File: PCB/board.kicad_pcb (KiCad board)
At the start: 2 copper layers, 161 parts, among them J1 Micro_SD_Card, J10 Conn_01x10, J11 Conn_01x02, J12 Conn_02x04_Odd_Even, J13 Conn_01x02, J14 Conn_01x02, J15 Conn_01x03, J16 Conn_01x02, J17 Conn_01x05, J18 Conn_01x04, J19 Conn_01x04, J2 Conn_ARM_JTAG_SWD_10, J20 Conn_01x02, J21 Conn_01x03, J22 Conn_02x04_Odd_Even, J23 Conn_01x04, J24 Conn_01x04, J25 Conn_01x02, J26 Conn_01x03, J27 Conn_02x04_Odd_Even, J28 Conn_01x04, J29 Conn_01x04, J3 USB_C_Receptacle_USB2.0_14P, J30 Conn_01x02, J31 Conn_01x03, J32 Conn_01x02, J33 Conn_01x02, J34 Conn_01x02, J35 Conn_01x02, J36 Conn_01x02, J37 Conn_01x02, J4 Conn_01x04, J5 Conn_01x04, J6 Conn_01x02, J7 Conn_01x03, J8 Conn_02x04_Odd_Even, J9 Conn_01x10, Q1 IRLML6402, Q2 NMOS, Q3 NMOS, Q4 NMOS, Q5 NMOS, Q6 NMOS, SW1 SW_Push, SW2 SW_Push, U1 STM32H743VITx, U2 AP7361C, U4 TMC Stepstick, U5 TMC Stepstick, U6 TMC Stepstick, U7 TMC Stepstick, U8 AP63203WU, Y2 25 MHz

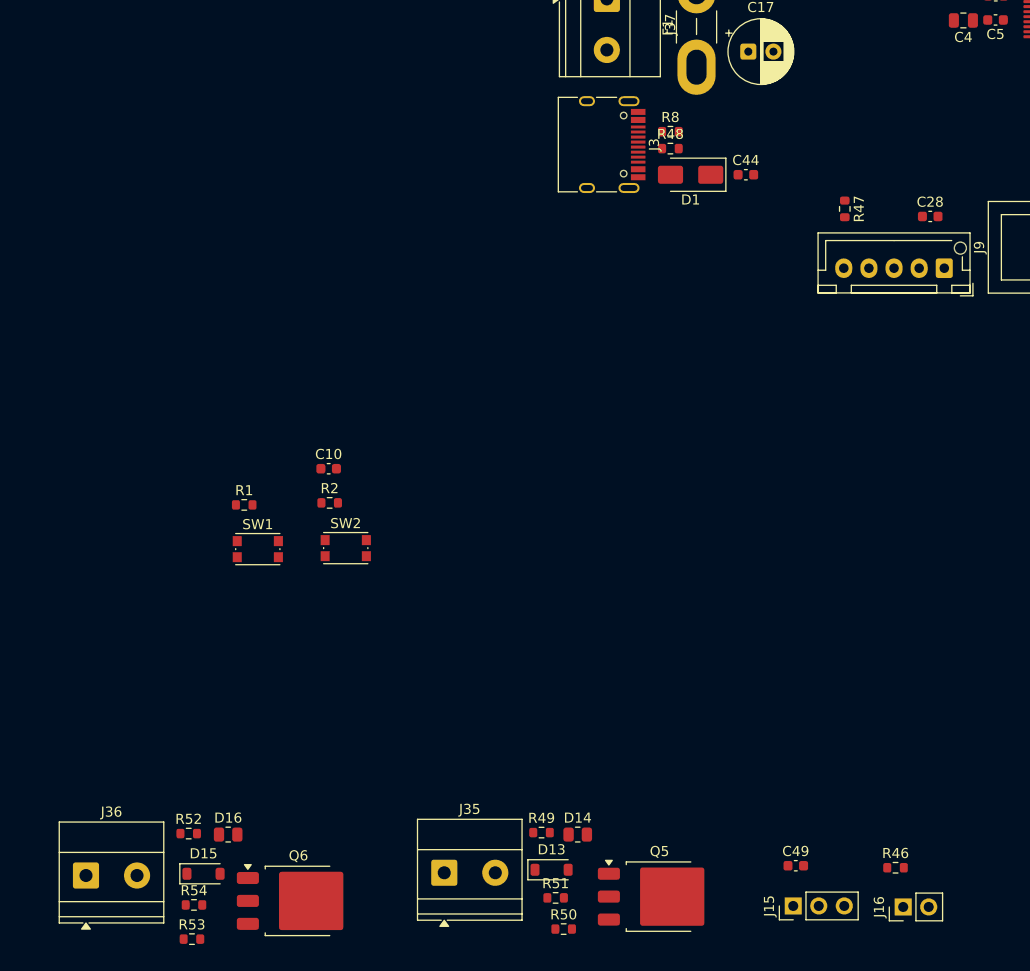
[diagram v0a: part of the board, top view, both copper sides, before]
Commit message: heaters
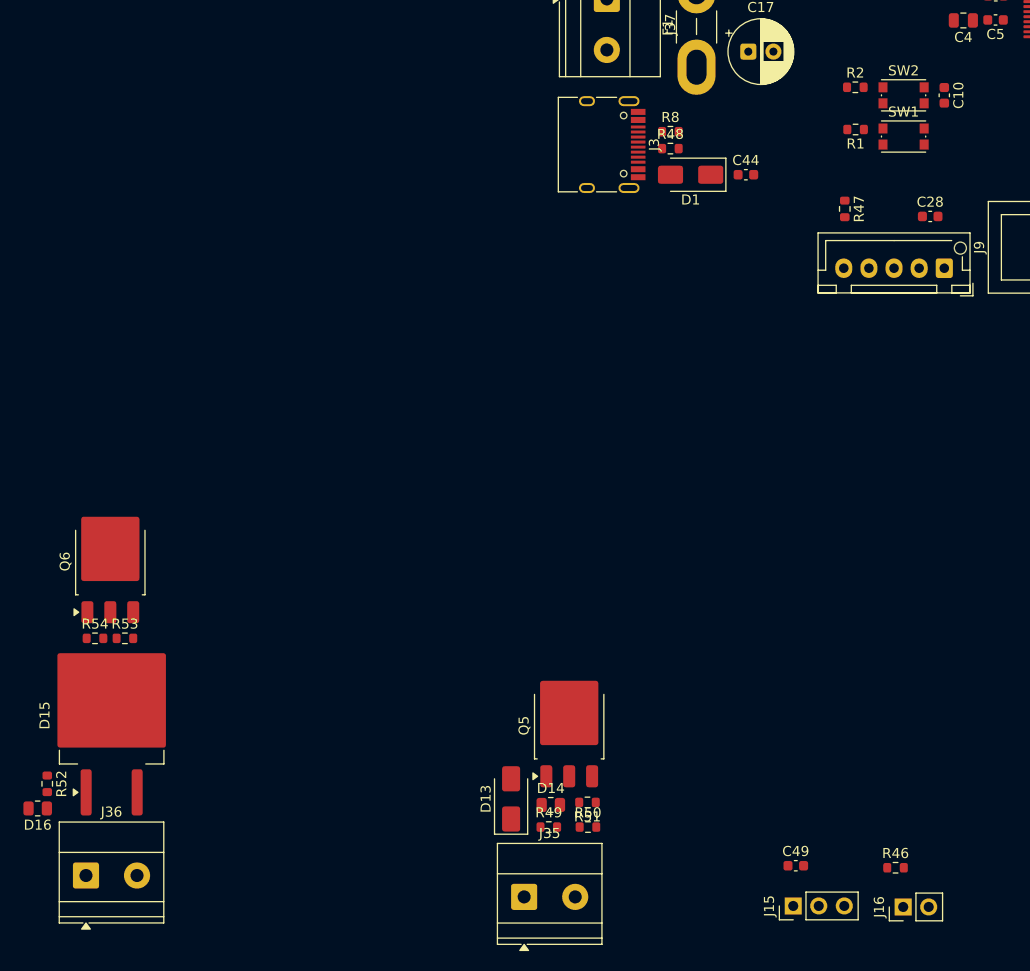
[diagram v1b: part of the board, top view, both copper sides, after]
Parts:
- D13: footprint Diode_SMD:D_SOD-123 -> Diode_SMD:D_SMA
- D15: footprint Diode_SMD:D_SOD-123 -> Package_TO_SOT_SMD:TO-263-2
- moved SW1 76.2 mm to (170.7, 107.8)
- moved C10 71.6 mm to (174.8, 103.8), turned to -90 degrees
- moved SW2 71.5 mm to (170.7, 103.8)
- moved R1 71.4 mm to (165.9, 107.2), turned to 180 degrees
- moved R2 66.7 mm to (165.9, 103.0)
- moved Q6 38.6 mm to (91.8, 150.1), turned to 90 degrees
- moved R53 30.7 mm to (93.2, 157.8)
- moved R54 28.3 mm to (90.3, 157.8)
- moved Q5 19.2 mm to (137.4, 166.5), turned to 90 degrees
- moved D16 19.1 mm to (84.5, 174.7), turned to 180 degrees
- moved D15 18.2 mm to (91.9, 165.4), turned to 90 degrees
- moved R52 14.9 mm to (85.5, 172.2), turned to -90 degrees
- moved R50 10.4 mm to (139.3, 176.6)
- moved R51 10.0 mm to (139.2, 174.1), turned to 180 degrees
- moved J35 8.30 mm to (132.9, 183.5)
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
